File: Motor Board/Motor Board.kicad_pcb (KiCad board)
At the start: 2 copper layers, 40 x 40 mm, 44 parts, among them J1 Programmer, J2 Gecko, J3 Gecko, J4 Conn_01x02_Socket, J5 Conn_01x02_Socket, Q1 BSS316NN, Q2 DMG2305UX-7, U2 PIC18F26K83, U3 MCP2562, U4 INA180, Y1 12MHz Crystal

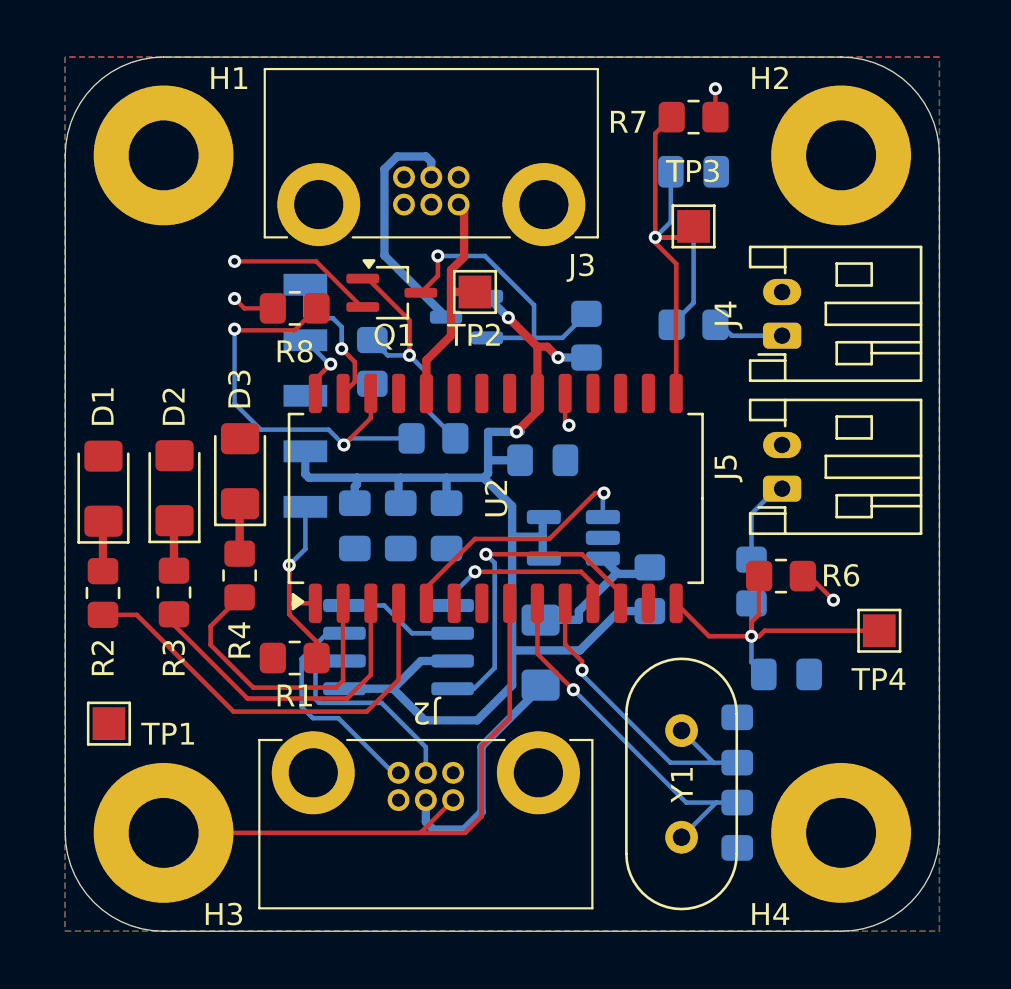
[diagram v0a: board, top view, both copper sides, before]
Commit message: redit layout
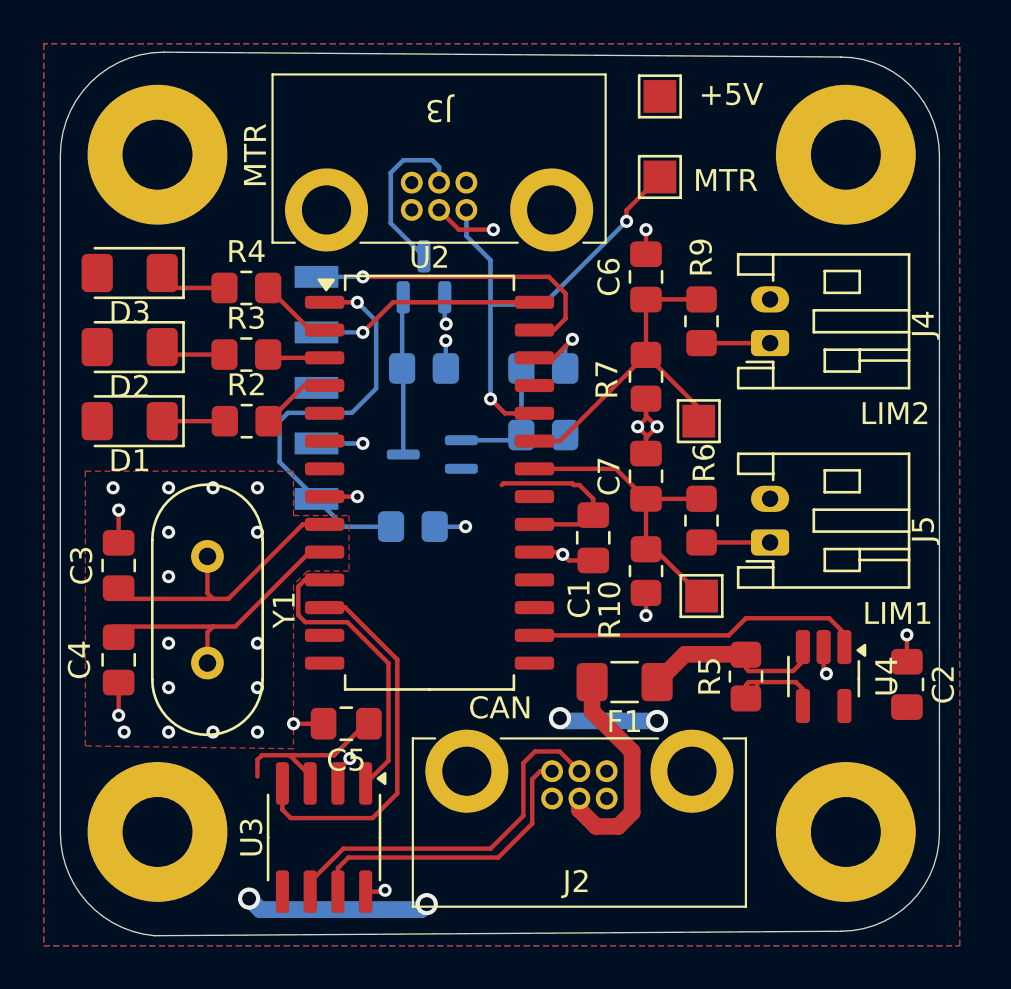
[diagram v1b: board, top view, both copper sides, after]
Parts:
- removed the C1 at (168.1, 62.7)
- removed the C1 at (170.2, 62.7)
- removed the R8 at (163.2, 52.8)
- removed the R8 at (176.6, 54.0)
- added C1: 0.1uF, Capacitor_SMD:C_0805_2012Metric_Pad1.18x1.45mm_HandSolder, F.Cu at (176.9, 63.2)
- added G***: LOGO, Team_Logo:Logo_Horizontal_Silkscreen_10mm, B.Cu at (174.5, 67.8)
- added R8: 10kR, Resistor_SMD:R_0805_2012Metric_Pad1.20x1.40mm_HandSolder, B.Cu at (169.2, 55.5)
- C2, C3, C4, C5, C6, C7, F1, R10, R5, R9, U3, U4: moved to F.Cu
- J1: footprint Canhw:PinSocket_5x2.54_SMD_90deg_952-3198-1-ND -> canhw:PinSocket_5x2.54_SMD_90deg_952-3198-1-ND
- J2, J3: footprint Canhw:connector_Harwin_G125–MG10605M4P -> canhw:connector_Harwin_G125–MG10605M4P
- Q1, R1: moved to B.Cu
- Y1: value 12MHz Crystal -> 12MHz Crystal
- moved TP1 38.2 mm to (180.0, 43.1), turned to 180 degrees
- moved C3 30.7 mm to (155.2, 64.5), turned to 90 degrees
- moved C4 28.5 mm to (155.2, 68.8), turned to -90 degrees
- moved Y1 25.2 mm to (159.3, 64.1), turned to -90 degrees
- moved C2 19.6 mm to (191.3, 70.0), turned to -90 degrees
- moved R4 13.2 mm to (161.0, 51.8), turned to 0 degrees
- moved U4 13.1 mm to (187.5, 69.6), turned to -90 degrees
- moved R7 12.1 mm to (179.3, 55.9), turned to -90 degrees
- moved R3 11.4 mm to (161.0, 54.9), turned to 0 degrees
- moved C7 11.1 mm to (179.3, 60.4), turned to 90 degrees
- moved D3 10.4 mm to (155.7, 51.1), turned to 180 degrees
- moved R2 10.2 mm to (161.1, 57.9), turned to 0 degrees
- moved TP2 9.96 mm to (180.0, 46.7)
- moved U3 9.35 mm to (164.6, 77.0), turned to -90 degrees
- moved C5 9.06 mm to (165.6, 71.8), turned to 180 degrees
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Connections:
- U2 pad 14: /LIM_1 -> unconnected-(U2-RC3-Pad14)
- U2 pad 15: /LIM_2 -> unconnected-(U2-RC4-Pad15)
- U2 pad 16: unconnected-(U2-RC5-Pad16) -> /CURR_SENS
- U2 pad 22: unconnected-(U2-RB1-Pad22) -> /LIM_1
- U2 pad 23: unconnected-(U2-RB2-Pad23) -> /LIM_2
- U2 pad 5: /CURR_SENS -> unconnected-(U2-RA3-Pad5)
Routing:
- net GND: track 46.1 -> 24.2 mm, vias 5 -> 29
- net +5V: track 60.8 -> 39.5 mm, vias 3 -> 8
- net Net-(U2-RA2): track 19.5 -> 3.24 mm
- net /MTR_ON: track 19.5 -> 3.65 mm, vias 2 -> 1
- net /MTR_IN: track 10.6 -> 22.8 mm, vias 0 -> 2
- net Net-(U2-RA1): track 14.6 -> 2.64 mm
- net /~{MCLR}: track 8.94 -> 19.2 mm
- net Net-(U2-RA0): track 13.3 -> 3.38 mm
- net /LIM_2: track 24.8 -> 15.8 mm, vias 1 -> 0
- net /ICSPCLK: track 6.80 -> 14.5 mm
- net /ICSPDAT: track 3.25 -> 10.5 mm
- net /CANL: track 10.0 -> 17.0 mm
- net Net-(Q1-D): track 13.8 -> 7.23 mm, vias 1 -> 0
- net Net-(Q1-G): track 11.2 -> 5.90 mm, vias 1 -> 0
- net /CAN_TX: track 8.49 -> 13.6 mm, vias 1 -> 0
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- added copper zone on F.Cu, net GND
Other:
- board size 40 x 40 mm -> 40.2 x 40.4 mm
- board text added: "+5V"
- board text added: "CAN"
- board text added: "LIM1"
- board text added: "LIM2"
- board text added: "MTR"
- board text added: "Motor Board Connor Stubbs 24-05-2024"
- board text added: "~{MCLR}"
- board text removed: "MCLR"
